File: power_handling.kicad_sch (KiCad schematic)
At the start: 60 parts, among them J1 FH34SRJ-16S-0.5SH_50_, SW1 MK-12C02 G1.5, U1 AP22802AW5-7, U2 FSUSB42MUX, U3 TPS62827DMQR, U4 TPS62065DSGR, U5 ME6211C18M5G-N

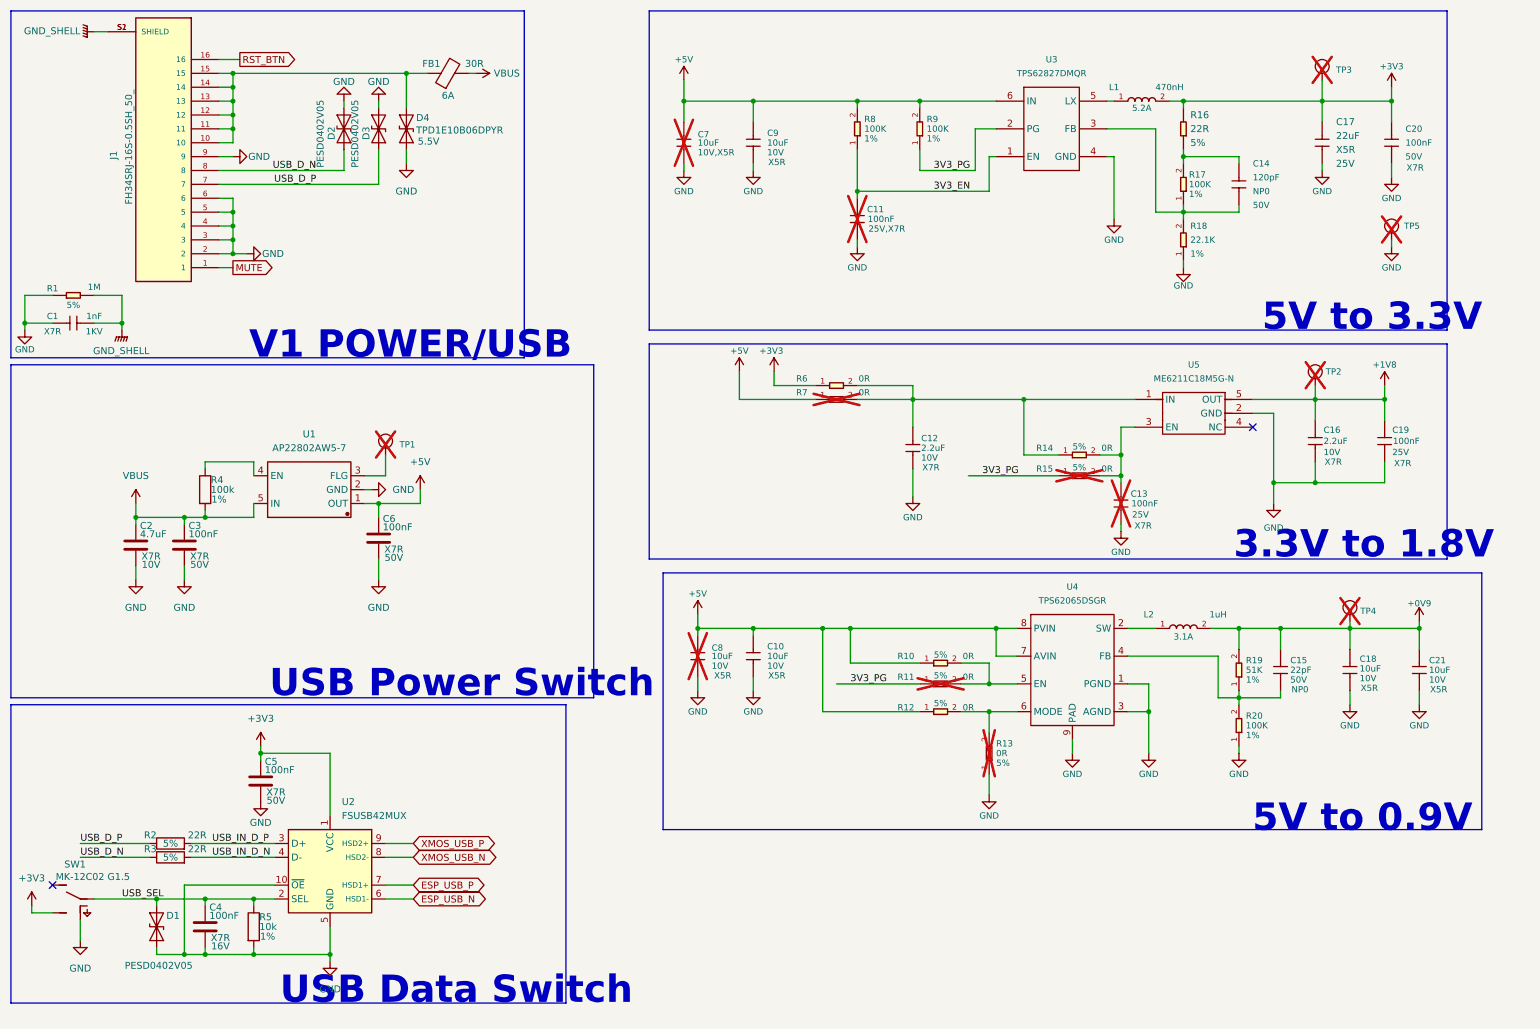
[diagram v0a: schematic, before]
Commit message: 1st test batch
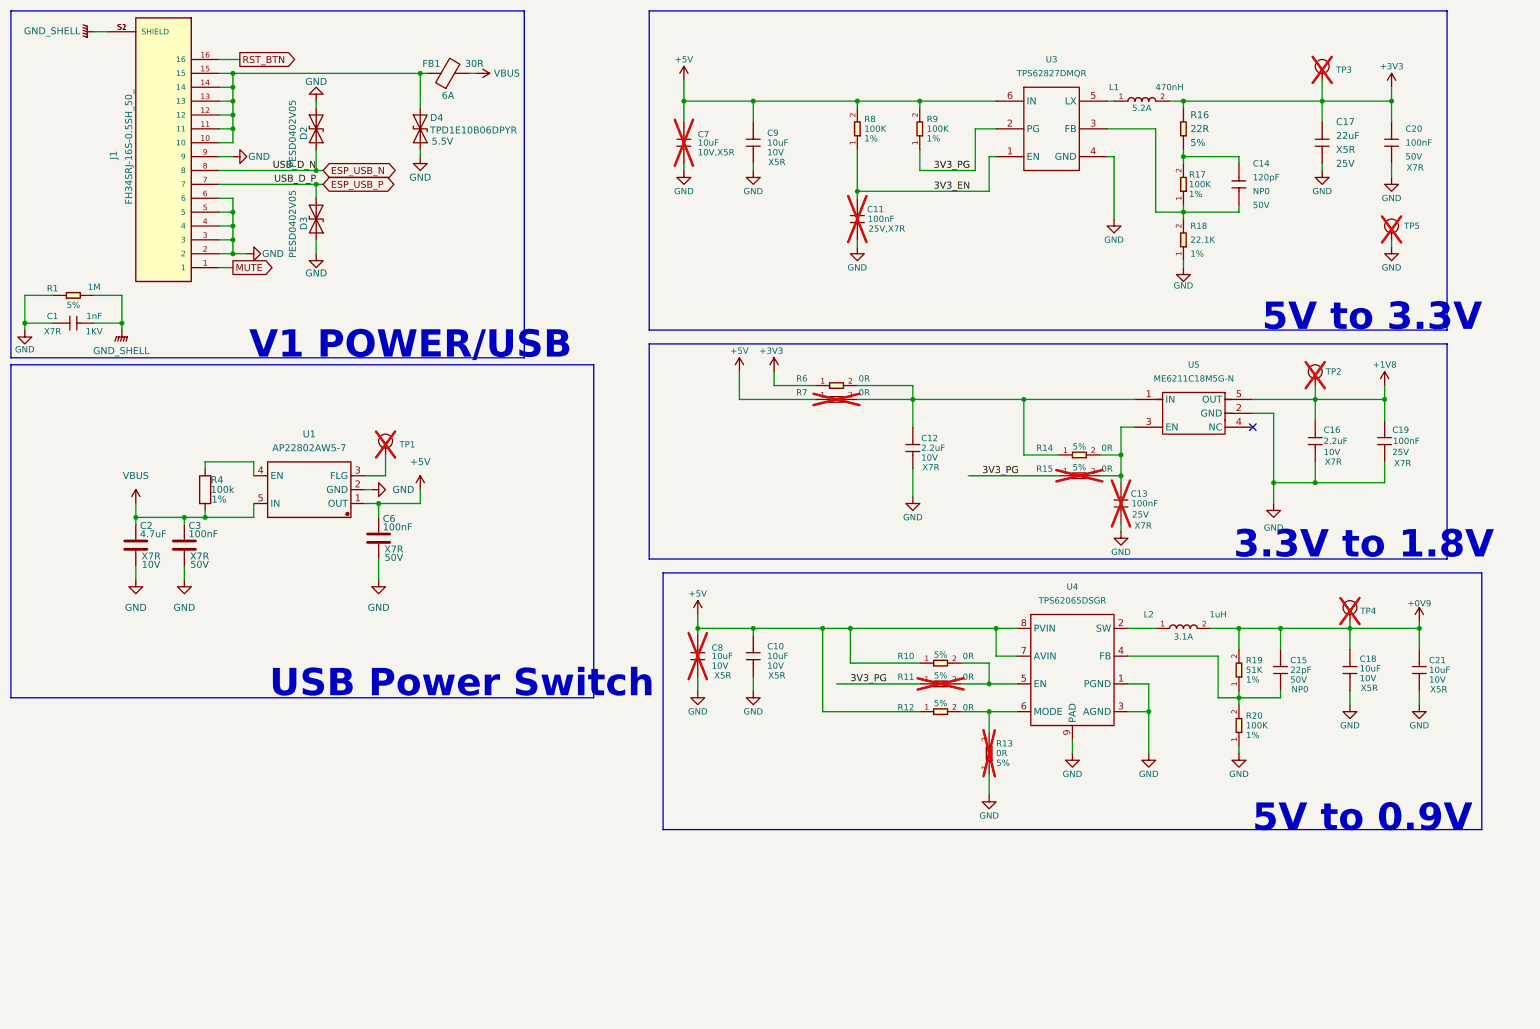
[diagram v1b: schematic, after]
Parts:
- removed C4: 100nF, Capacitor_SMD:C_0402_1005Metric, symbol Device:C
- removed C5: 100nF, Capacitor_SMD:C_0603_1608Metric, symbol Device:C
- removed D1: PESD0402V05, Diode_SMD:D_0402_1005Metric, symbol Diode:SZESD9B5.0ST5G
- removed R2, R3: 22R, Resistor_SMD:R_0402_1005Metric, symbol Device:R
- removed R5: 10k, Resistor_SMD:R_0402_1005Metric, symbol Device:R
- removed SW1: MK-12C02 G1.5, Onju:SW7-SMD-L6.7X2.7X3.2MM, symbol New_Library:MK-12C02_G1.5
- removed U2: FSUSB42MUX, Package_SO:MSOP-10_3x3mm_P0.5mm, symbol Interface_USB:FSUSB42MUX
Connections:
- net USB_D_N is gone; now on net ESP_USB_N: D2.2 (A2), J1.8
- net ESP_USB_P: now also D3.1 (A1), J1.7
- net GND: now also D3.2 (A2); no longer D3.1 (A1)
- removed net USB_D_P: D3.2 (A2), J1.7
- no-connect marks 2 -> 1
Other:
- note removed: "USB Data Switch"
- moved on the sheet: D2, D3, D4

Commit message: Production update
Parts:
- C1: Purchase-URL (none) -> https://www.lcsc.com/product-detail/C89334.html?s_z=n_2450A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
- C10, C18, C21, C9: Purchase-URL (none) -> https://www.lcsc.com/product-detail/C19702.html?s_z=n_CL10A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
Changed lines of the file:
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@@
 			)
 		)
+		(property "Purchase-URL" "https://www.lcsc.com/product-detail/C19702.html?s_z=n_CL10A106KP8NNNC"
+			(at 148.59 38.1 0)
+			(effects
+				(font
+					(size 1.27 1.27)
+				)
+				(hide yes)
+			)
+		)
 		(pin "2"
 		)
@@
 			)
 		)
+		(property "Purchase-URL" "https://www.lcsc.com/product-detail/C19702.html?s_z=n_CL10A106KP8NNNC"
+			(at 257.81 134.62 0)
+			(effects
+				(font
+					(size 1.27 1.27)
+				)
+				(hide yes)
+			)
+		)
 		(pin "1"
 		)
@@
 			)
 		)
+		(property "Purchase-URL" "https://www.lcsc.com/product-detail/C19702.html?s_z=n_CL10A106KP8NNNC"
+			(at 148.59 132.08 0)
+			(effects
+				(font
+					(size 1.27 1.27)
+				)
+				(hide yes)
+			)
+		)
 		(pin "2"
 		)
@@
 			)
 		)
+		(property "Purchase-URL" "https://www.lcsc.com/product-detail/C89334.html?s_z=n_2450AT18A100E"
+			(at 24.13 71.12 90)
+			(effects
+				(font
+					(size 1.27 1.27)
+				)
+				(hide yes)
+			)
+		)
 		(pin "1"
 		)
@@
 			(at 270.51 134.62 0)
 			(effects
+				(font
+					(size 1.27 1.27)
+				)
+				(hide yes)
+			)
+		)
+		(property "Purchase-URL" "https://www.lcsc.com/product-detail/C19702.html?s_z=n_CL10A106KP8NNNC"
+			(at 270.51 134.62 0)
+			(effects
